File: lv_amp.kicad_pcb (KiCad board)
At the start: 2 copper layers, 139.7 x 88.9 mm, 80 parts, among them J1 AudioJack2, J2 Jack-DC, J3 AudioJack2, Q1 Q_NMOS_DGS, U1 ECC83, U2 TL072, U3 ECC83, U4 ECC83, U5 MAX1771xSA

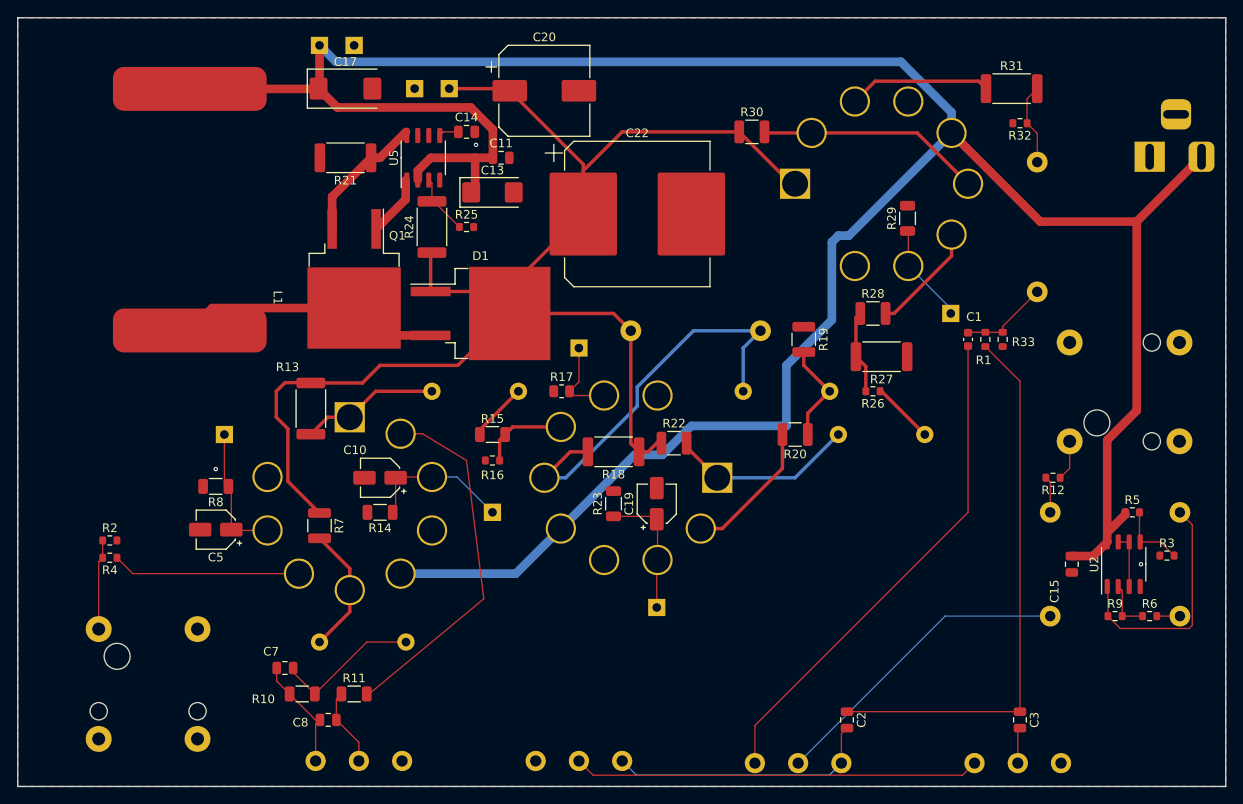
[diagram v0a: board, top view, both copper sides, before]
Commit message: tighter layout
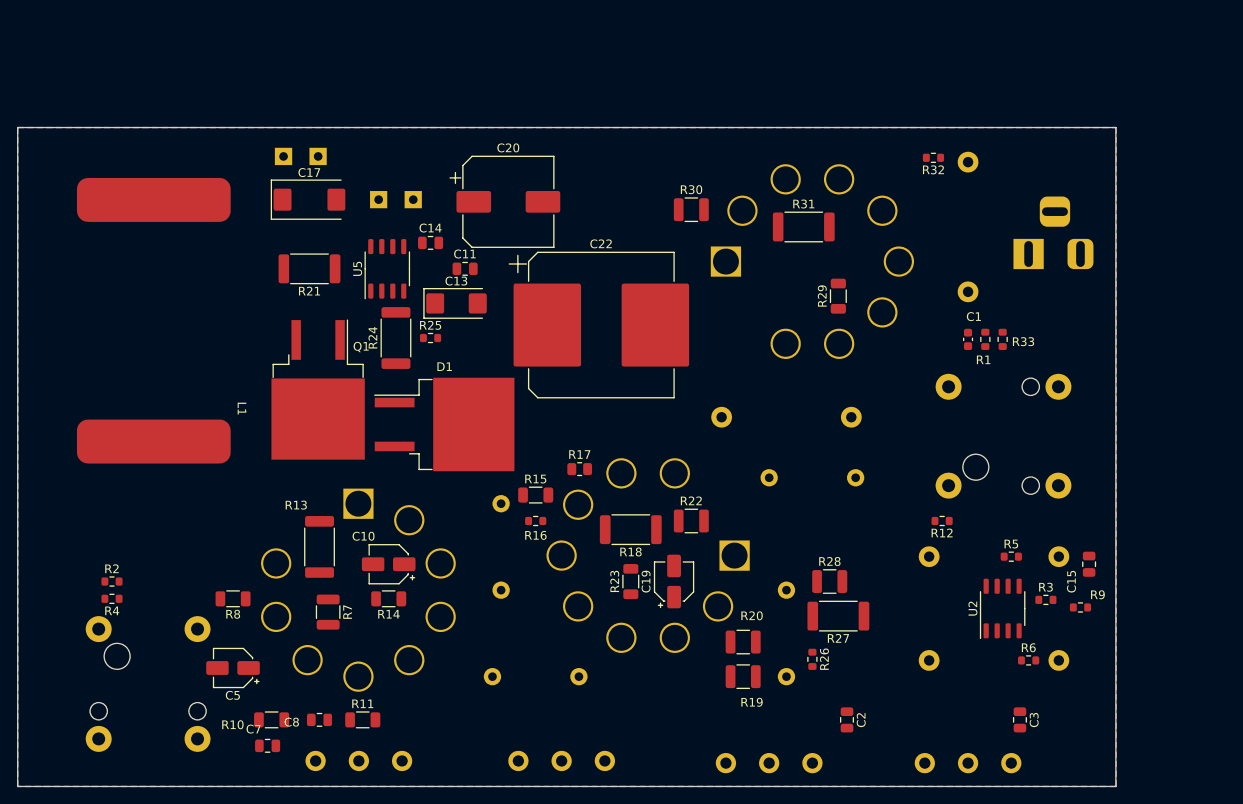
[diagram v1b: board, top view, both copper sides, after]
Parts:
- removed TP1, TP5, TP6, TP7, TP8: TestPoint, TestPoint:TestPoint_THTPad_2.0x2.0mm_Drill1.0mm
- moved R19 39.6 mm to (122.0, 127.0), turned to 0 degrees
- moved R26 31.8 mm to (130.0, 125.0), turned to -90 degrees
- moved R28 31.4 mm to (132.0, 116.0)
- moved R27 30.4 mm to (133.0, 120.0)
- moved C6 30.3 mm to (103.0, 127.0), turned to 180 degrees
- moved R31 28.9 mm to (129.0, 75.0)
- moved C21 28.6 mm to (127.0, 127.0), turned to 90 degrees
- moved R20 24.7 mm to (122.0, 123.0)
- moved J2 18.0 mm to (155.0, 78.1)
- moved C5 16.1 mm to (63.0, 126.0)
- moved R13 16.0 mm to (73.0, 112.0)
- moved C12 15.3 mm to (94.0, 107.0), turned to -90 degrees
- moved C4 14.9 mm to (143.5, 125.1)
- moved C9 14.9 mm to (158.5, 113.1)
- moved J3 14.9 mm to (145.8, 104.9)
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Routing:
- net +12V: track 315.1 -> 0.00 mm
- net HT: track 162.6 -> 0.00 mm
- net Net-(C2-Pad1): track 63.9 -> 0.00 mm
- net Net-(C1-Pad2): track 58.4 -> 0.00 mm
- net /u3ap: track 47.4 -> 0.00 mm
- net Net-(RV2-Pad2): track 47.0 -> 0.00 mm
- net Net-(R11-Pad2): track 42.1 -> 0.00 mm
- net Net-(C4-Pad1): track 36.2 -> 0.00 mm
- net Net-(C2-Pad2): track 30.9 -> 0.00 mm
- net /d1a: track 30.2 -> 0.00 mm
- net Net-(C9-Pad1): track 27.6 -> 0.00 mm
- net /u4ap: track 26.0 -> 0.00 mm
- net Net-(R4-Pad1): track 21.8 -> 0.00 mm
- net /u3bp: track 21.5 -> 0.00 mm
- net Net-(C10-Pad1): track 17.1 -> 0.00 mm
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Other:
- board size 139.7 x 88.9 mm -> 127 x 76.2 mm

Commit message: flipsies
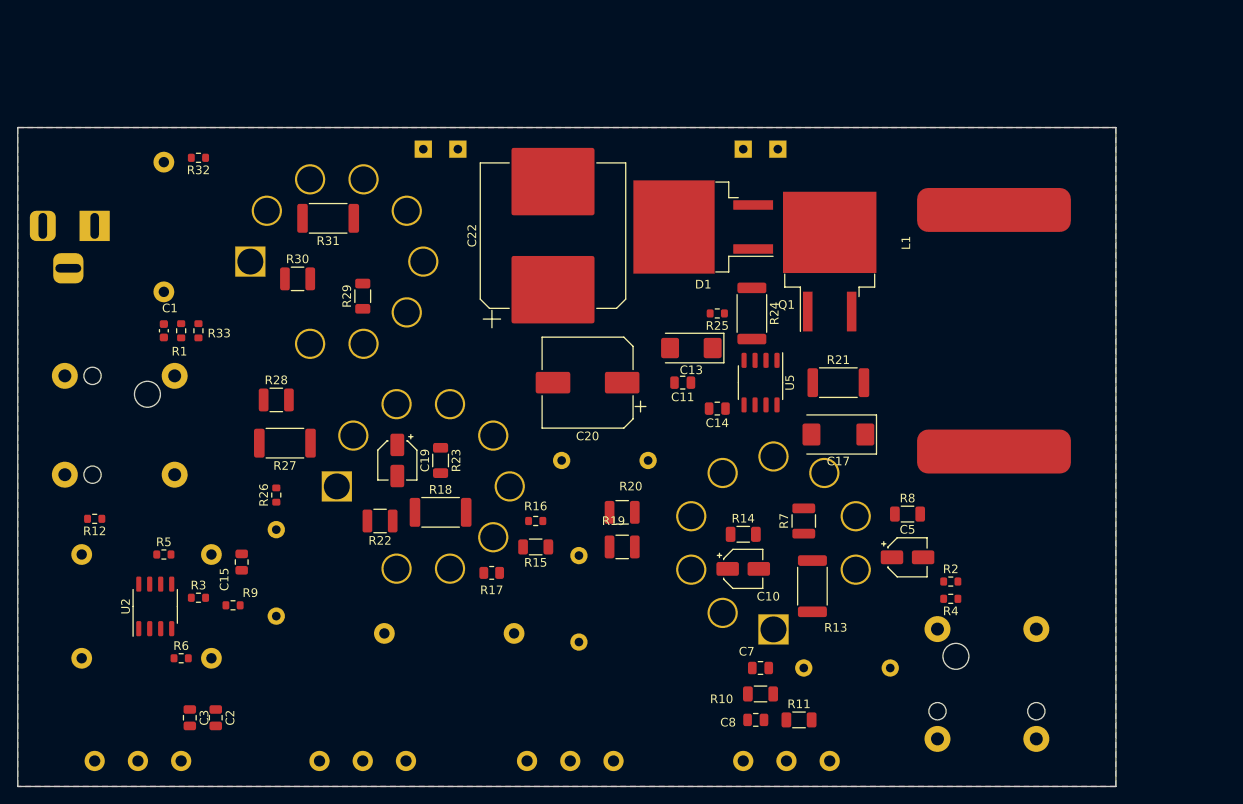
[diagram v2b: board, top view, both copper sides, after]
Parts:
- moved J2 108.0 mm to (47.0, 74.9), turned to 0 degrees
- moved C15 98.0 mm to (64.0, 113.8)
- moved C4 98.0 mm to (45.5, 124.9)
- moved C9 98.0 mm to (60.5, 112.9)
- moved R12 98.0 mm to (47.0, 108.8)
- moved R3 98.0 mm to (59.0, 117.9)
- moved R5 98.0 mm to (55.0, 112.9)
- moved R6 98.0 mm to (57.0, 124.9)
- moved R9 98.0 mm to (63.0, 118.8)
- moved U2 98.0 mm to (54.0, 118.9)
- moved L1 97.2 mm to (151.0, 87.0), turned to 90 degrees
- moved J1 97.0 mm to (144.5, 121.5)
- moved R2 97.0 mm to (146.0, 116.0)
- moved R4 97.0 mm to (146.0, 118.0)
- moved C3 96.0 mm to (58.0, 131.8)
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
